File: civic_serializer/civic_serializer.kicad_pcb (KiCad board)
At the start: 2 copper layers, 65 x 30 mm, 36 parts, among them IC1 DS90UB925QSQX_NOPB, J1 GPIO, U1 AMS1117-3.3

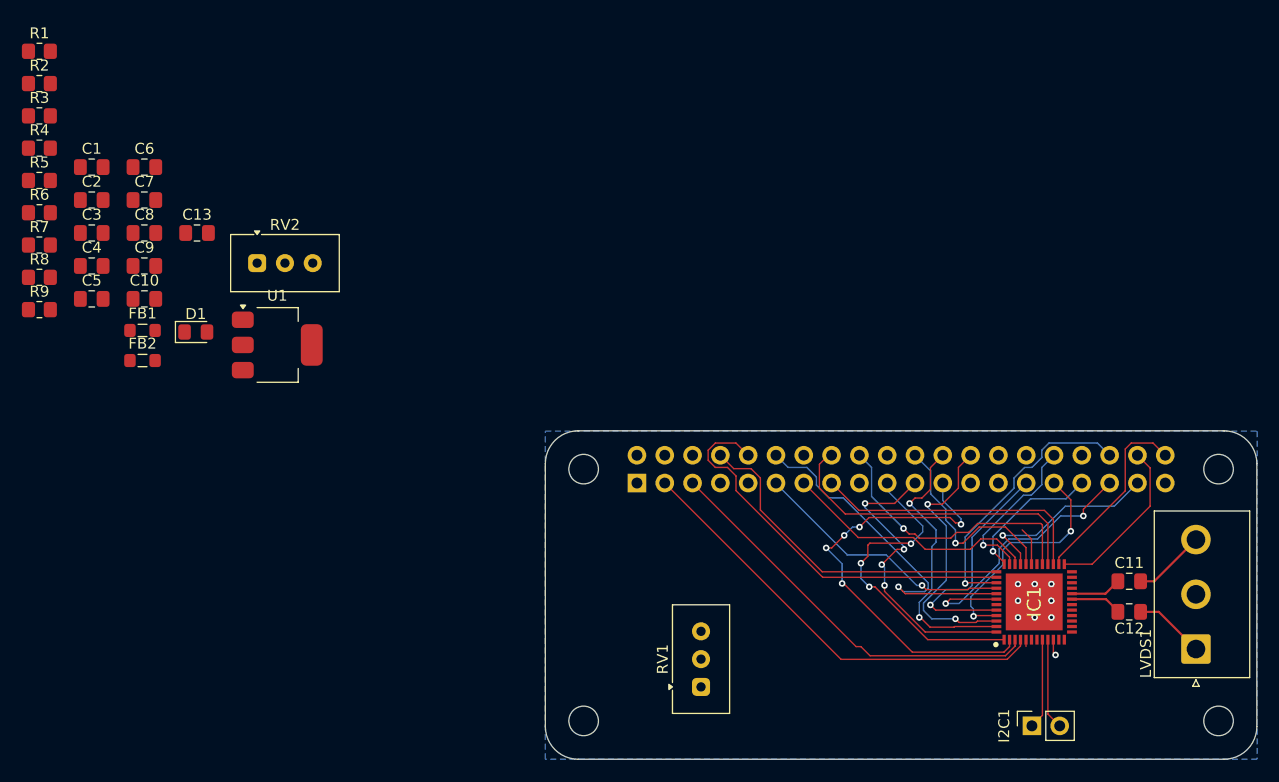
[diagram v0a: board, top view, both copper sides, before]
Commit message: - layout finished
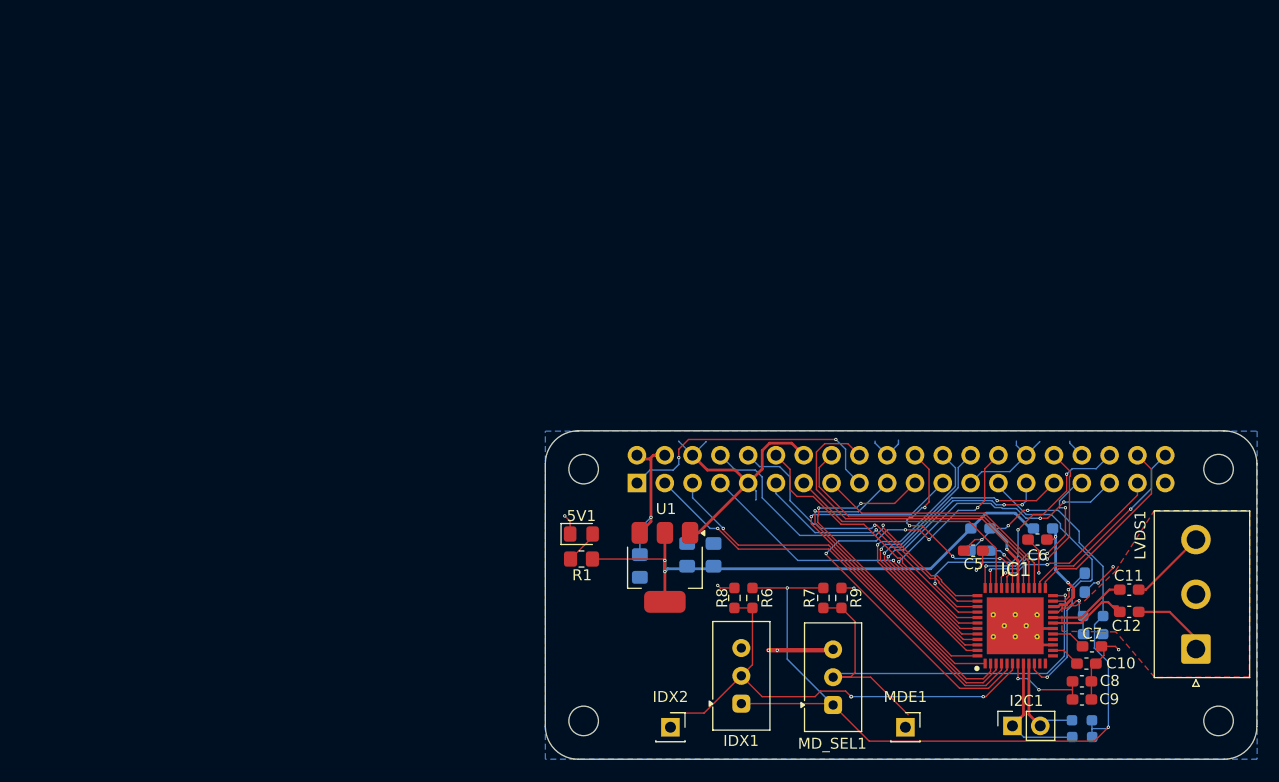
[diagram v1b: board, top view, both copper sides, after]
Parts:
- removed D1: LED, LED_SMD:LED_0805_2012Metric_Pad1.15x1.40mm_HandSolder
- removed RV1, RV2: R_Potentiometer_Trim, Potentiometer_THT:Potentiometer_Vishay_T93YA_Vertical
- added 5V1: LED, LED_SMD:LED_0805_2012Metric_Pad1.15x1.40mm_HandSolder, F.Cu at (103.3, 79.4)
- added IDX1: R_Potentiometer_Trim, Potentiometer_THT:Potentiometer_Vishay_T93YA_Vertical, F.Cu at (117.9, 94.9)
- added IDX2: TestPoint, Connector_PinSocket_2.54mm:PinSocket_1x01_P2.54mm_Vertical, F.Cu at (111.4, 97.1)
- added MDE1: TestPoint, Connector_PinSocket_2.54mm:PinSocket_1x01_P2.54mm_Vertical, F.Cu at (132.9, 97.1)
- added MD_SEL1: R_Potentiometer_Trim, Potentiometer_THT:Potentiometer_Vishay_T93YA_Vertical, F.Cu at (126.3, 95.0)
- C1, C13: footprint Capacitor_SMD:C_0805_2012Metric_Pad1.18x1.45mm_HandSolder -> Capacitor_SMD:C_0603_1608Metric_Pad1.08x0.95mm_HandSolder; moved to B.Cu
- C10, C11, C12, C5, C6, C7, C8, C9: footprint Capacitor_SMD:C_0805_2012Metric_Pad1.18x1.45mm_HandSolder -> Capacitor_SMD:C_0603_1608Metric_Pad1.08x0.95mm_HandSolder
- C2, C3, C4: moved to B.Cu
- FB1, FB2: footprint Inductor_SMD:L_0805_2012Metric_Pad1.05x1.20mm_HandSolder -> Inductor_SMD:L_0603_1608Metric_Pad1.05x0.95mm_HandSolder; moved to B.Cu
- R2, R3, R4, R5: footprint Resistor_SMD:R_0805_2012Metric_Pad1.20x1.40mm_HandSolder -> Resistor_SMD:R_0603_1608Metric_Pad0.98x0.95mm_HandSolder; moved to B.Cu
- R6, R7, R8, R9: footprint Resistor_SMD:R_0805_2012Metric_Pad1.20x1.40mm_HandSolder -> Resistor_SMD:R_0603_1608Metric_Pad0.98x0.95mm_HandSolder
- moved R4 109.4 mm to (149.0, 98.0)
- moved R2 107.8 mm to (150.0, 86.9)
- moved R5 107.2 mm to (149.0, 96.4)
- moved C1 98.3 mm to (149.3, 83.9), turned to -90 degrees
- moved C7 95.7 mm to (149.9, 89.7)
- moved C8 94.9 mm to (149.0, 92.9)
- moved R3 94.7 mm to (139.8, 81.0), turned to 180 degrees
- moved C9 94.4 mm to (149.0, 94.5)
- moved C10 92.3 mm to (149.4, 91.3)
- moved C13 89.7 mm to (150.0, 88.6)
- moved C6 88.4 mm to (145.0, 79.9), turned to 180 degrees
- moved C5 83.7 mm to (139.1, 81.0)
- moved FB2 83.7 mm to (145.5, 78.9)
- moved FB1 78.7 mm to (139.8, 78.9)
- moved R7 78.5 mm to (125.4, 85.3), turned to 90 degrees
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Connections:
- net Net-(IC1-DOUT+) renamed DOUT+
- net Net-(IC1-DOUT-) renamed DOUT-
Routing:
- net VDDIO: track 0.00 -> 97.9 mm, vias 0 -> 6
- net GND: track 0.00 -> 81.0 mm, vias 8 -> 10
- net 3V3: track 0.00 -> 50.2 mm, vias 0 -> 2
- net MODE_SEL: track 0.00 -> 47.2 mm, vias 0 -> 1
- net DE: track 0.63 -> 44.9 mm, vias 0 -> 4
- net IDX: track 0.00 -> 43.7 mm, vias 0 -> 2
- net B0: track 0.00 -> 29.1 mm, vias 0 -> 1
- net +3V3: track 0.00 -> 25.5 mm, vias 0 -> 2
- net PCLK: track 1.48 -> 26.9 mm
- net +5V: track 0.00 -> 14.0 mm, vias 0 -> 1
- net VDD33: track 0.00 -> 10.1 mm, vias 0 -> 2
- net B2: track 21.5 -> 30.5 mm
- net G3: track 36.9 -> 28.0 mm, vias 0 -> 1
- net CAPL12: track 0.00 -> 8.43 mm, vias 0 -> 2
- net G7: track 25.5 -> 32.9 mm, vias 2 -> 3
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- added copper zone on F.Cu, net GND
